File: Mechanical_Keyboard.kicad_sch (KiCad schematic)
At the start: 124 parts, among them SW1 MX, SW10 MX, SW11 MX, SW12 MX, SW13 MX, SW14 MX, SW15 MX, SW16 MX, SW17 MX, SW18 MX, SW19 MX, SW2 MX, SW20 MX, SW21 MX, SW22 MX, SW23 MX, SW24 MX, SW25 MX, SW26 MX, SW27 MX, SW28 MX, SW29 MX, SW3 MX, SW30 MX, SW31 MX, SW32 MX, SW33 MX, SW34 MX, SW35 MX, SW36 MX, SW37 MX, SW38 MX, SW39 MX, SW4 MX, SW40 MX, SW41 MX, SW42 MX, SW43 MX, SW44 MX, SW46 MX, SW47 MX, SW48 MX, SW49 MX, SW5 MX, SW51 MX, SW52 MX, SW53 MX, SW54 MX, SW56 MX, SW57 MX, SW58 MX, SW59 MX, SW6 MX, SW61 MX, SW62 MX, SW63 MX, SW64 MX, SW66 MX, SW67 MX, SW7 MX, SW8 MX, SW9 MX

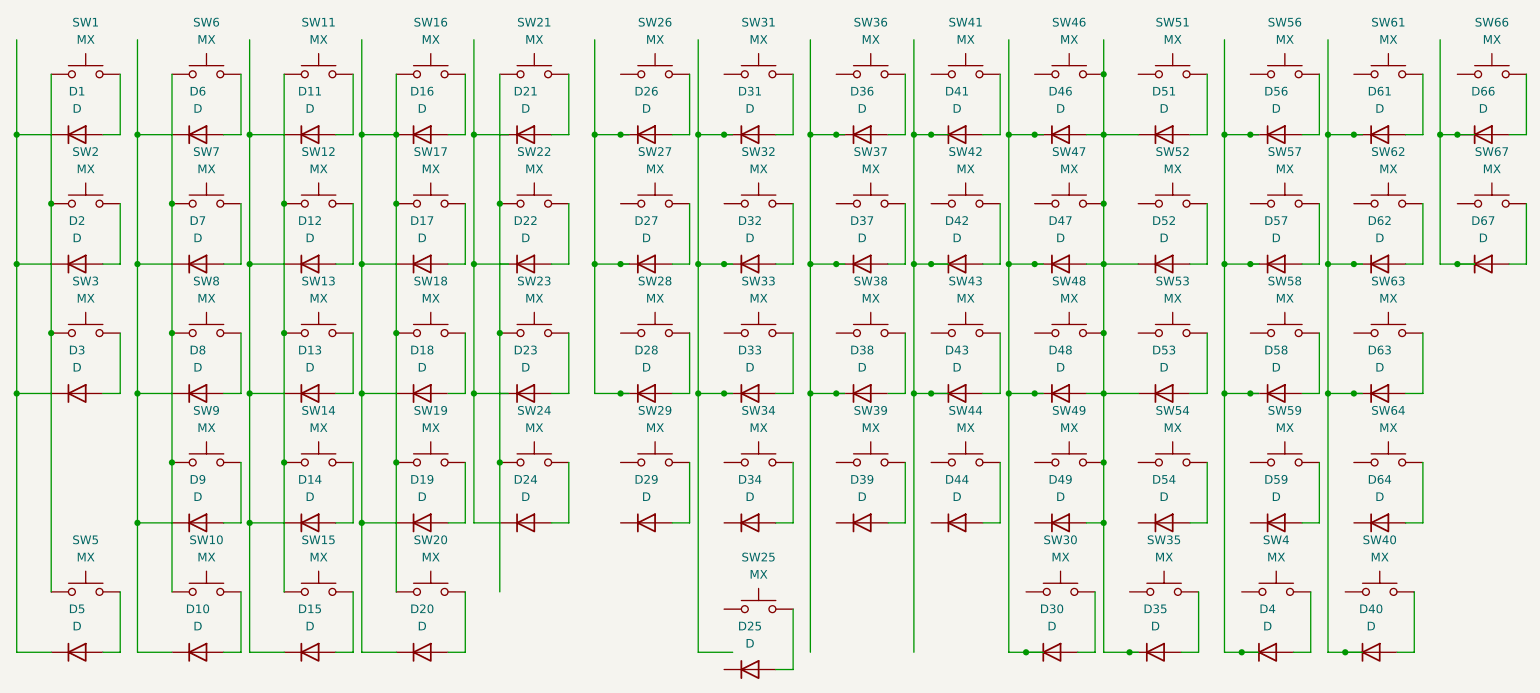
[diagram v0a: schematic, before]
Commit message: Add files via upload
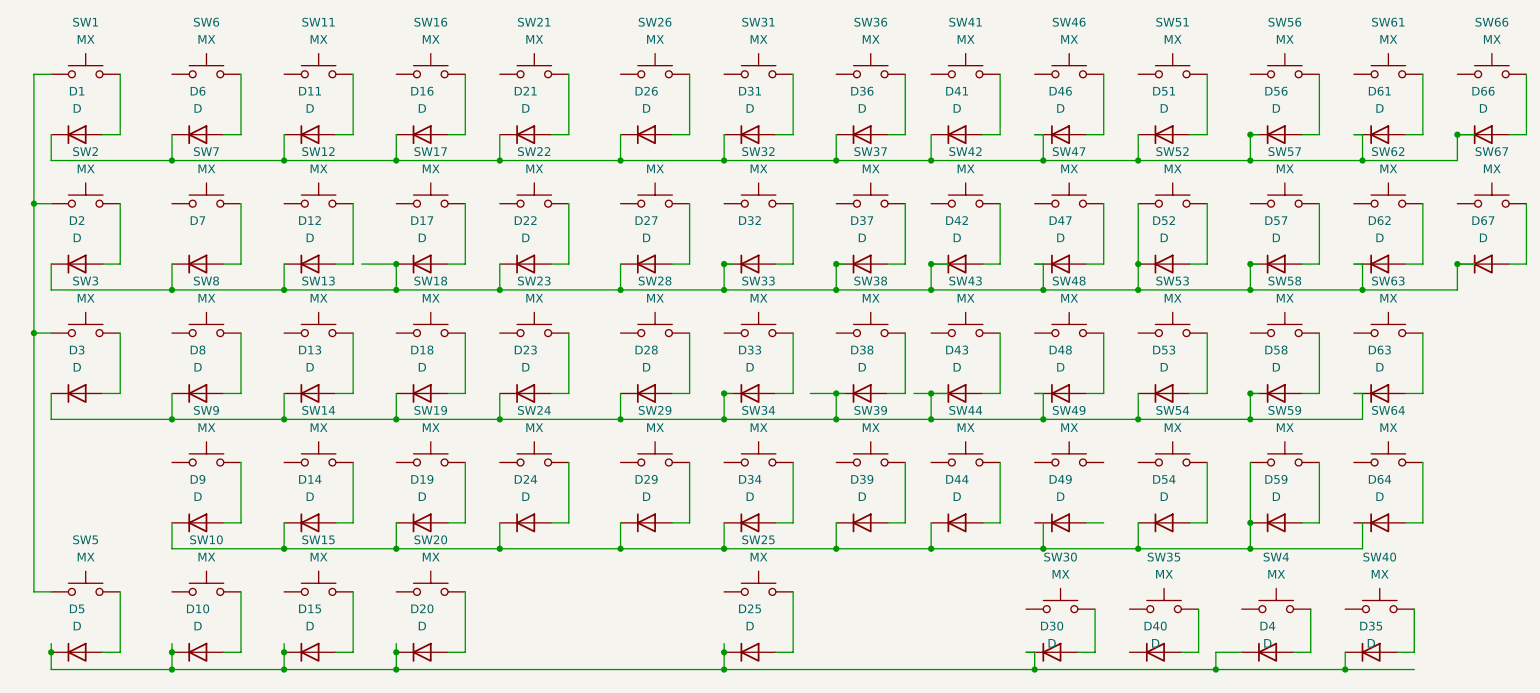
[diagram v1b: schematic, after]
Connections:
- net at D59.1 (K): now also D14.1 (K), D19.1 (K), D24.1 (K), D29.1 (K), D34.1 (K), D39.1 (K), D44.1 (K), D54.1 (K), D9.1 (K), SW59.1
- net at D35.2 (A): now also SW40.2; no longer SW35.2
- net at D22.1 (K): now also D12.1 (K), D17.1 (K), D2.1 (K), D27.1 (K), D32.1 (K), D37.1 (K), D42.1 (K), D47.1 (K), D52.1 (K), D57.1 (K), D62.1 (K), D67.1 (K), D7.1 (K), SW52.1
- net at D66.1 (K): now also D1.1 (K), D11.1 (K), D16.1 (K), D21.1 (K), D26.1 (K), D31.1 (K), D36.1 (K), D41.1 (K), D46.1 (K), D51.1 (K), D56.1 (K), D6.1 (K), D61.1 (K); no longer D67.1 (K)
- net at D25.1 (K): now also D10.1 (K), D15.1 (K), D20.1 (K), D30.1 (K), D35.1 (K), D4.1 (K), D5.1 (K)
- net at D40.2 (A): now also SW35.2; no longer SW40.2
- net at D23.1 (K): now also D13.1 (K), D18.1 (K), D28.1 (K), D3.1 (K), D33.1 (K), D38.1 (K), D43.1 (K), D48.1 (K), D53.1 (K), D58.1 (K), D63.1 (K), D8.1 (K)
- new net: D48.2 (A), SW48.2
- new net: D46.2 (A), SW46.2
- new net: D47.2 (A), SW47.2
- now unconnected: D40.1 (K), D49.2 (A), SW10.1, SW11.1, SW12.1, SW13.1, SW14.1, SW15.1, SW16.1, SW17.1, SW18.1, SW19.1, SW20.1, SW21.1, SW22.1, SW23.1, SW24.1, SW49.2, SW6.1, SW7.1, SW8.1, SW9.1
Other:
- moved on the sheet: D25, SW25, SW30, SW35, SW4, SW40
